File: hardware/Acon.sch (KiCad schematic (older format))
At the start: 12 parts, among them U1 AD620, U2 REF1004-2.5

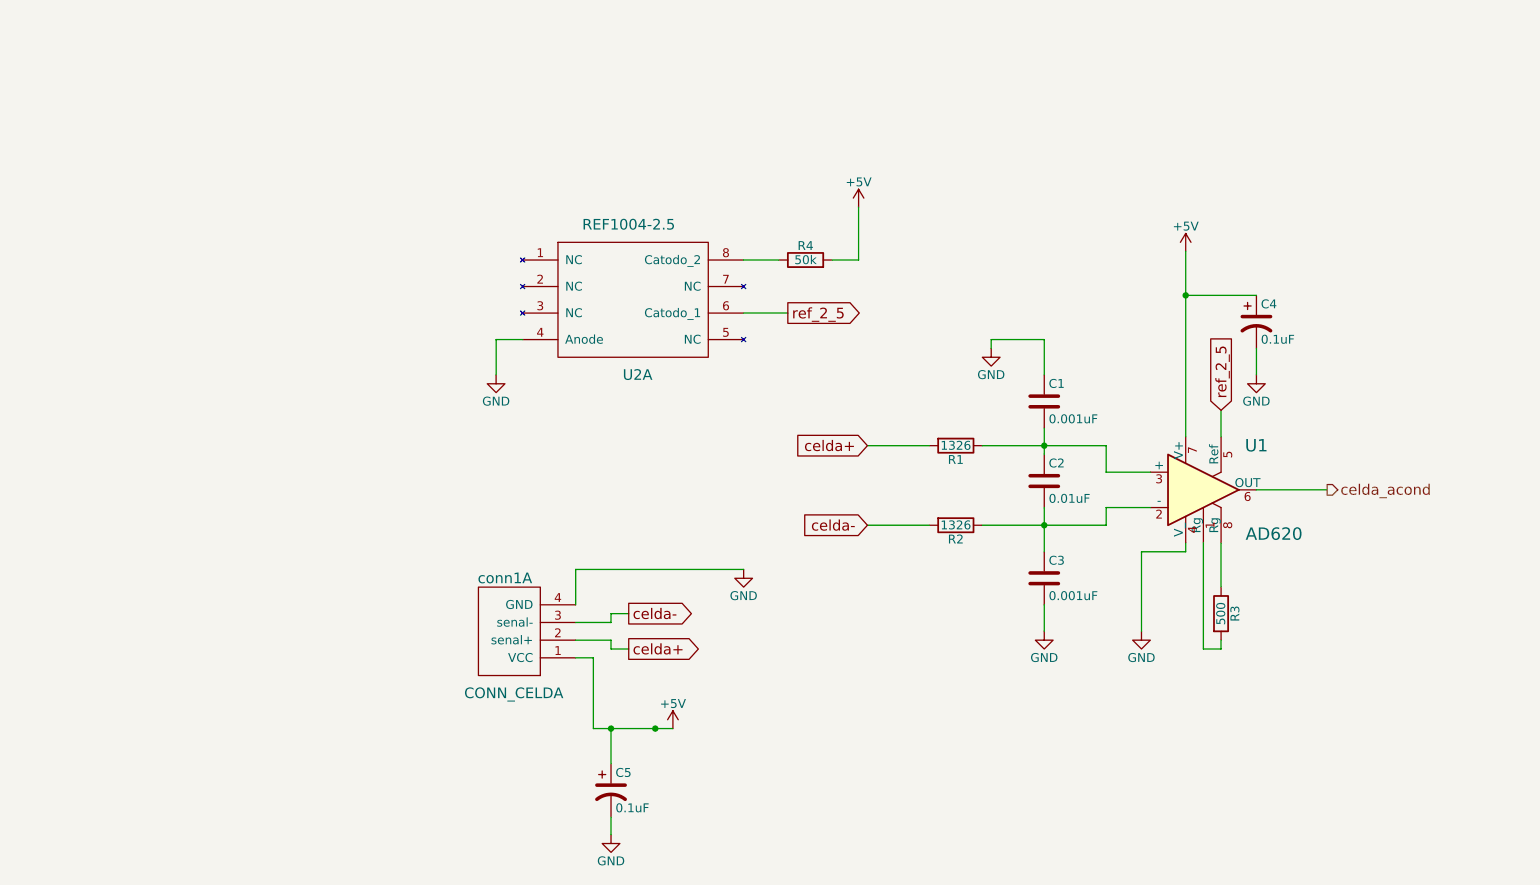
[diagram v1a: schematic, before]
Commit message: Se realizan correcciones al esquematico.
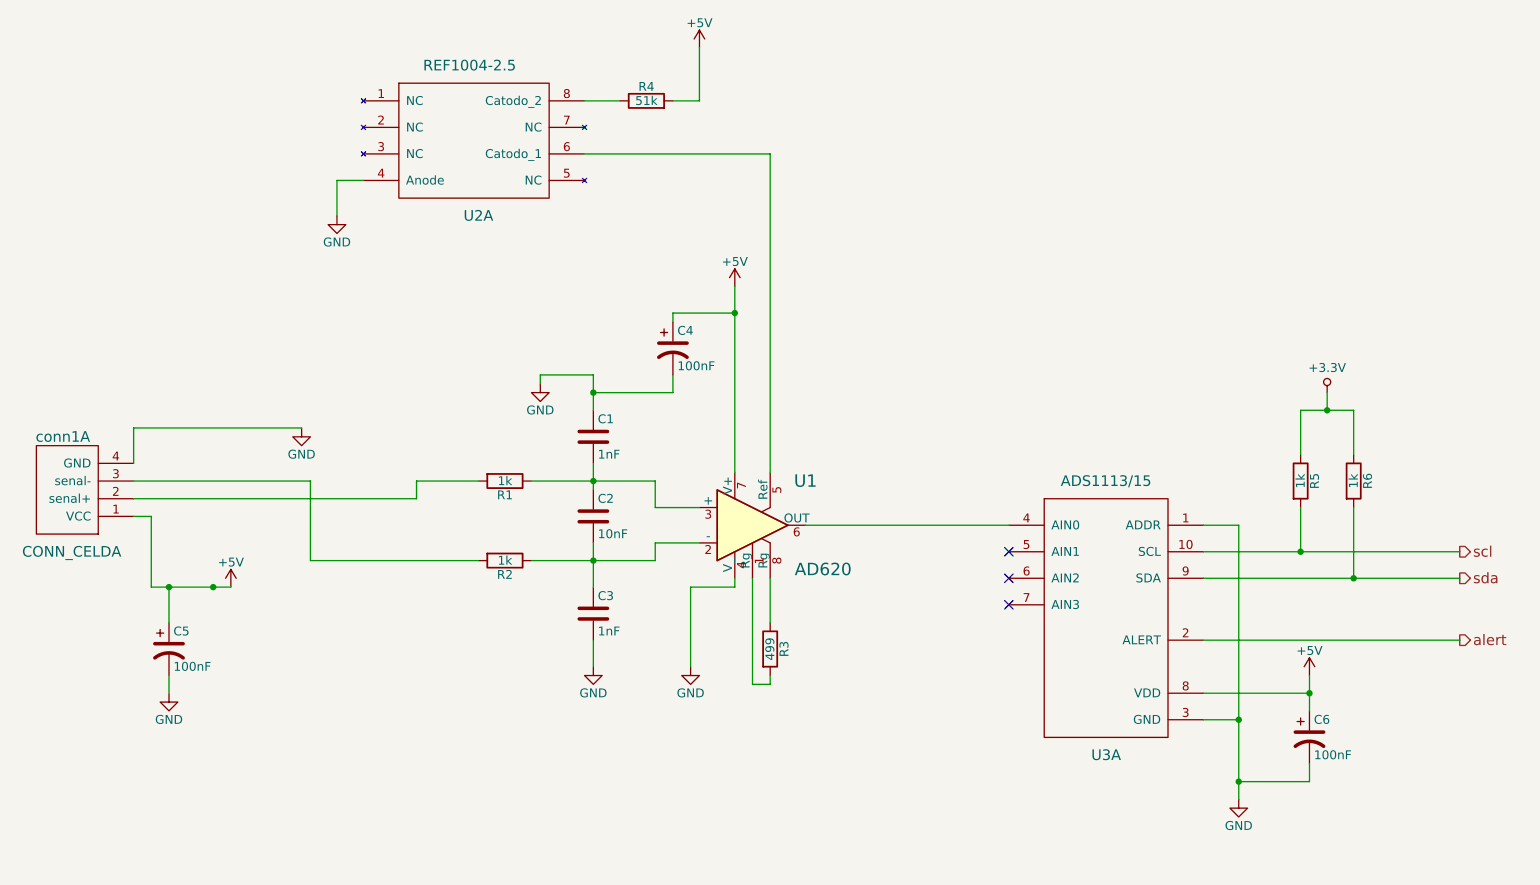
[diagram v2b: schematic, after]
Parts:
- added C6: 100nF, celda:C_0805_HandSoldering, symbol CP1
- added R5, R6: 1k, celda:R_1206_HandSoldering, symbol R
- added U3: ADS1113/15, celda:TSSOP-10_3x3mm_Pitch0.5mm, symbol ADS1113/15
- C1, C3: value 0.001uF -> 1nF; footprint ej2cese:C_0603_HandSoldering -> celda:C_0603_HandSoldering
- C2: value 0.01uF -> 10nF; footprint ej2cese:C_0603_HandSoldering -> celda:C_0603_HandSoldering
- C4, C5: value 0.1uF -> 100nF; footprint Capacitors_SMD:C_0805 -> celda:C_0805_HandSoldering
- R1, R2: value 1326 -> 1k; footprint ej2cese:R_1206_HandSoldering -> celda:R_1206_HandSoldering
- R3: value 500 -> 499; footprint ej2cese:R_1206_HandSoldering -> celda:R_1206_HandSoldering
- R4: value 50k -> 51k; footprint ej2cese:R_1206_HandSoldering -> celda:R_1206_HandSoldering
- U1, U2: footprint SMD_Packages:SOIC-8-N -> celda:SOIC-8
- conn1: footprint Connect:bornier4 -> celda:bornier4
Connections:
- net +5V: now also C6.1, U3.8 (VDD)
- net GND: now also C6.2, U3.1 (ADDR), U3.3 (GND)
- net celda+: no longer names the net of R1.2, conn1.2 (senal+)
- net celda-: no longer names the net of R2.2, conn1.3 (senal-)
- net celda_acond: no longer names the net of U1.6 (OUT)
- net celda_acond: now also U3.4 (AIN0)
- net ref_2_5: no longer names the net of U1.5 (Ref), U2.6 (Catodo_1)
- new net +3.3V: R5.1, R6.1
- new net alert: U3.2 (ALERT)
- new net scl: R5.2, U3.10 (SCL)
- new net sda: R6.2, U3.9 (SDA)
- no-connect marks 0 -> 3
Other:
- moved on the sheet: C1, C2, C3, C4, C5, R1, R2, R3, R4, U1, U2A, conn1A
